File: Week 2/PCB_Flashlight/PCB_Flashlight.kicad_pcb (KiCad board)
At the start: 2 copper layers, 50 x 10 mm, 18 parts, among them Q1 T2N7002AK,LM, SW1 ON, SW2 BLINK, U1 LTC6995-1, U2 MCP1799T-5002H/TT

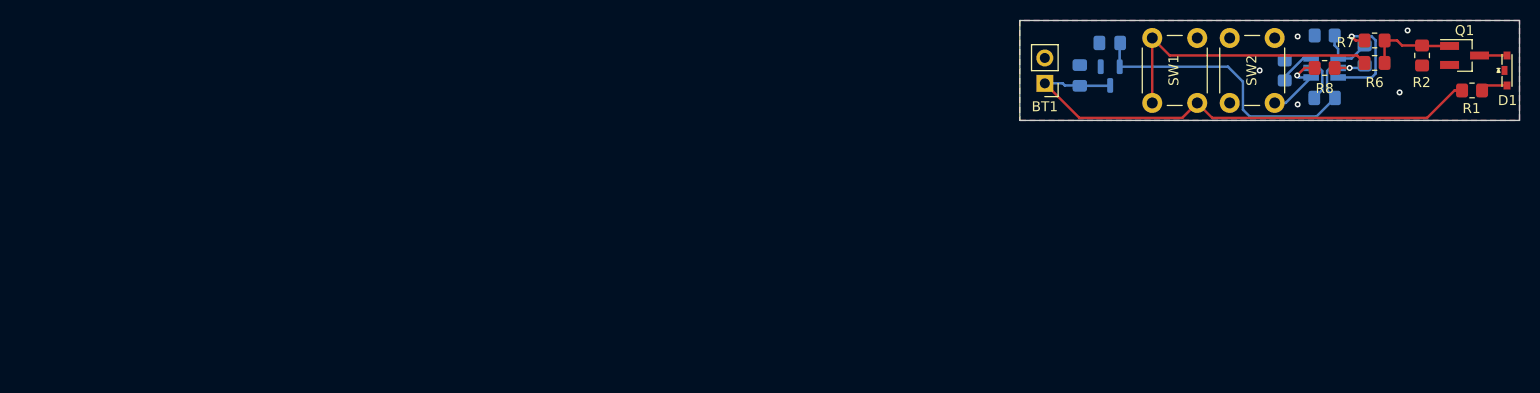
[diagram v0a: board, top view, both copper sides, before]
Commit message: Make the routing less horrendous
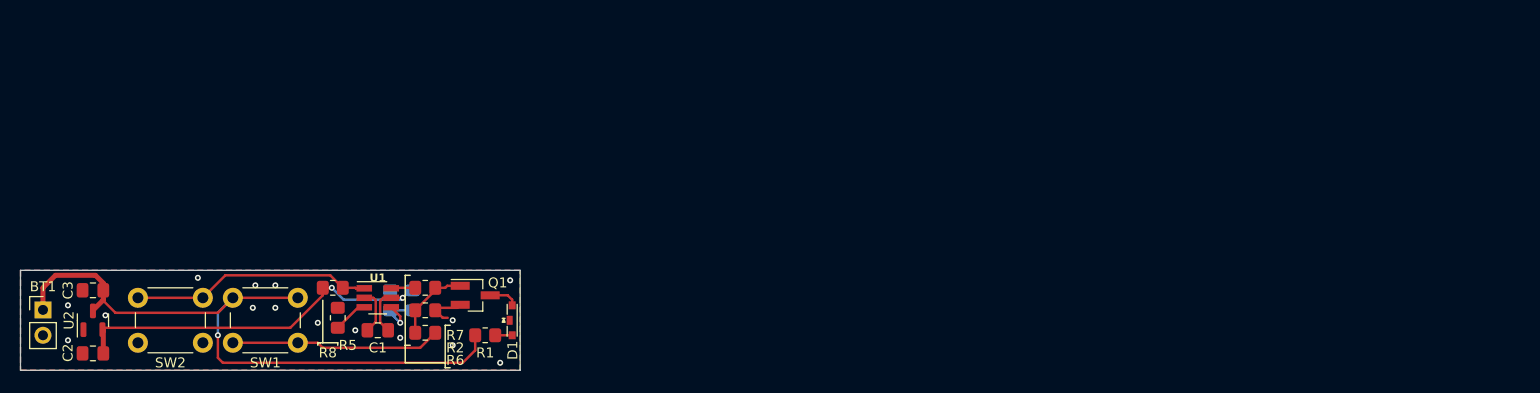
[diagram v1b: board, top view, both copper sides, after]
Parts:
- C1, C2, C3, R5, U1, U2: moved to F.Cu
- moved C2 106.4 mm to (57.2, 148.3)
- moved SW2 105.5 mm to (68.2, 147.2), turned to 180 degrees
- moved U2 104.7 mm to (57.2, 145.0), turned to 90 degrees
- moved R2 103.0 mm to (90.5, 144.0), turned to 0 degrees
- moved BT1 102.8 mm to (52.2, 144.0), turned to 0 degrees
- moved D1 102.6 mm to (99.2, 145.0)
- moved Q1 101.9 mm to (95.5, 142.5)
- moved R1 101.7 mm to (96.5, 146.5)
- moved R8 101.7 mm to (81.2, 141.8), turned to 0 degrees
- moved C3 101.1 mm to (57.2, 142.0), turned to 180 degrees
- moved SW1 99.9 mm to (71.2, 142.8), turned to 0 degrees
- moved R6 98.8 mm to (90.5, 146.2), turned to 180 degrees
- moved R3 98.4 mm to (89.2, 143.0), turned to -90 degrees
- moved R7 98.2 mm to (90.5, 141.8)
- moved R5 97.9 mm to (81.8, 144.8)
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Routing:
- net +9V: track 52.2 -> 68.5 mm, vias 0 -> 1
- net /BLINK_nON: track 8.25 -> 24.1 mm, vias 1 -> 0
- net Net-(U1-OUT): track 11.3 -> 2.42 mm, vias 1 -> 0
- net Net-(R6-Pad1): track 28.8 -> 21.1 mm
- net +5V: track 36.9 -> 42.2 mm, vias 1 -> 2
- net GND: track 4.25 -> 8.88 mm, vias 5 -> 15
- net /LED_ON: track 8.98 -> 7.91 mm
- net Net-(D1-A): track 2.71 -> 1.70 mm
- net Net-(U1-DIV): track 5.63 -> 5.84 mm, vias 0 -> 1
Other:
- board text added: "Designed by Jasper Rubin in 2023"
- board text added: "PCB_FLASHLIGHT REV0"
